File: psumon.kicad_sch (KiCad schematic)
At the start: 4 parts, among them U1 INA260

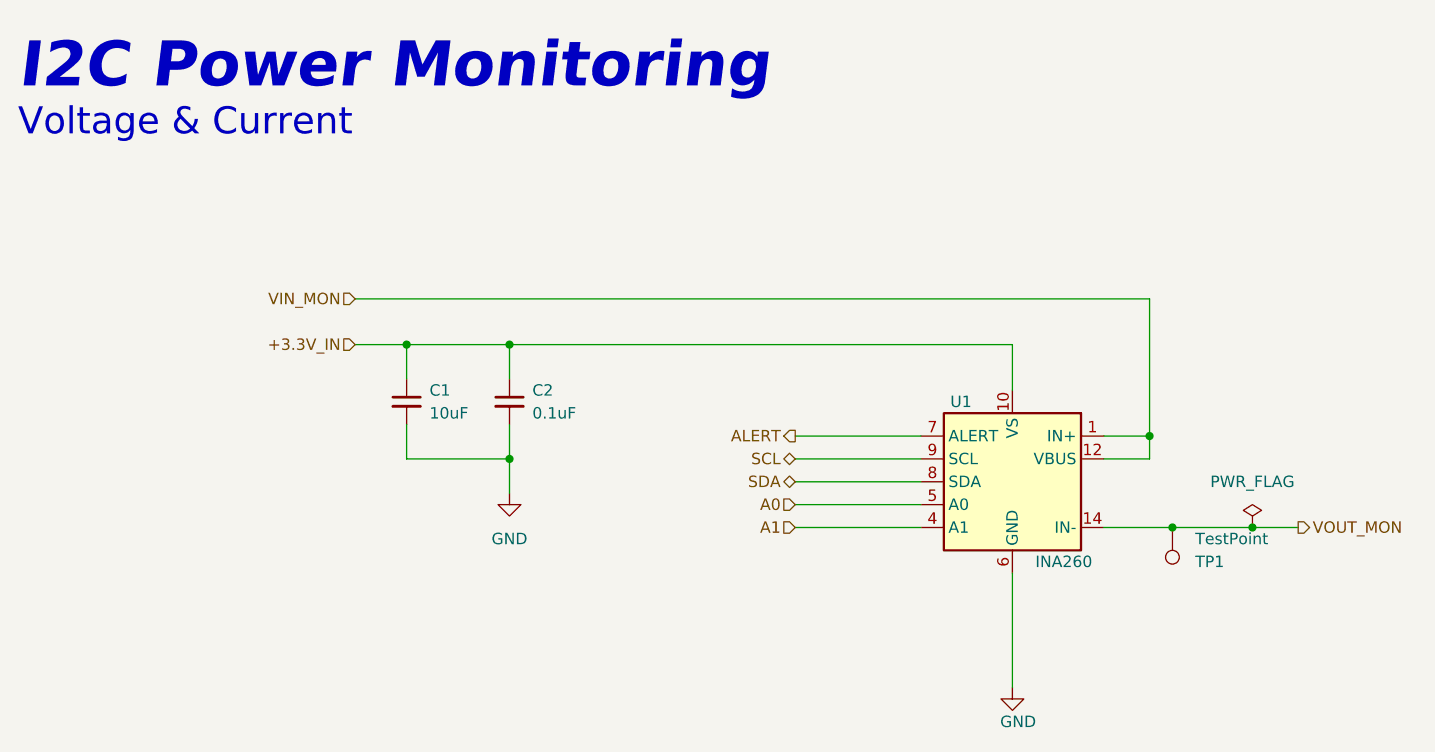
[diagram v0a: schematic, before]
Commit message: leds
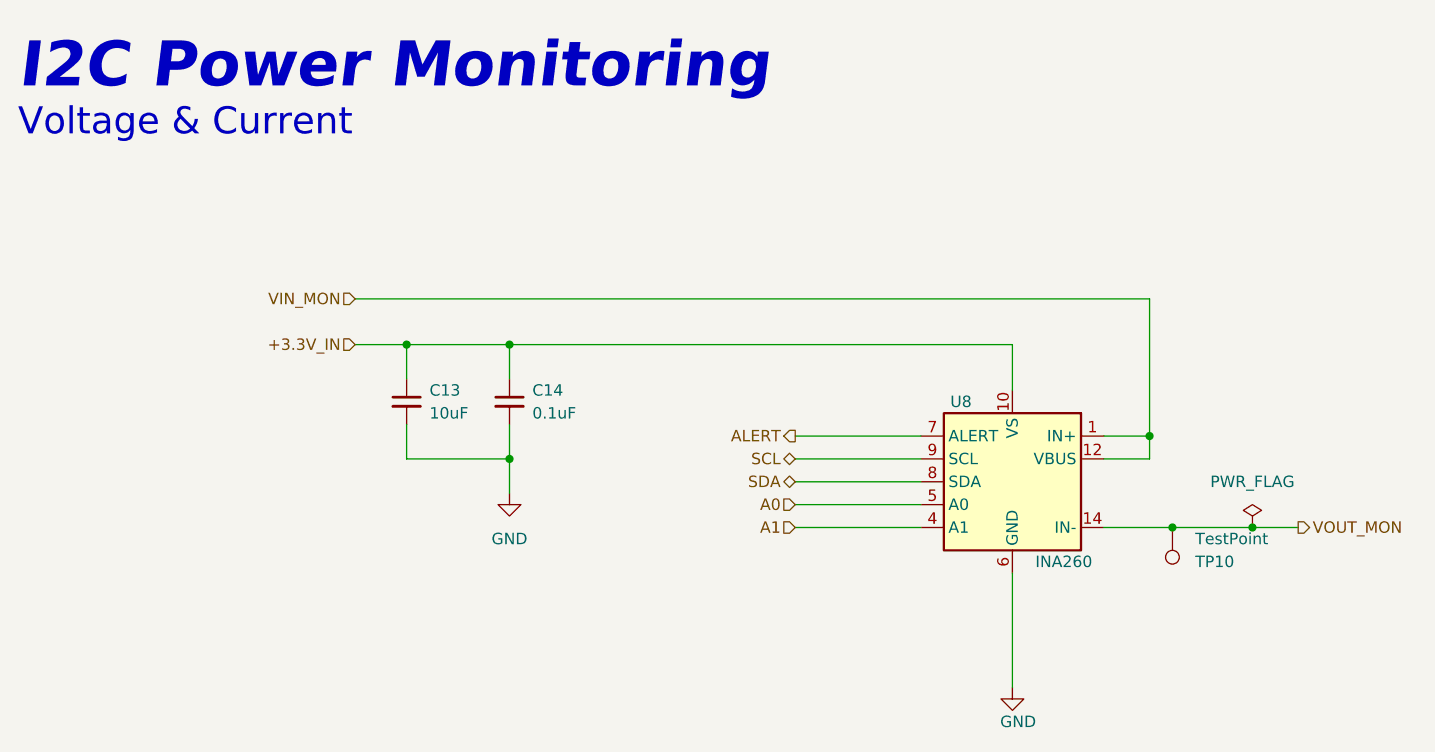
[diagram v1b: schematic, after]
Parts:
- renumbered C1 to C13, C2 to C14, TP1 to TP10, U1 to U8
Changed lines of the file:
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@@
   (symbol (lib_id "power:GND") (at 125.73 90.17 0)
     (in_bom yes) (on_board yes)
-    (property "Reference" "#PWR03" (id 0) (at 125.73 96.52 0)
+    (property "Reference" "#PWR023" (id 0) (at 125.73 96.52 0)
       (effects (font (size 1.27 1.27)) hide)
     )
@@
   (symbol (lib_id "Device:C_Small") (at 58.42 58.42 0)
     (in_bom yes) (on_board yes) (fields_autoplaced)
-    (property "Reference" "C1" (id 0) (at 60.96 57.1562 0)
+    (property "Reference" "C13" (id 0) (at 60.96 57.1562 0)
       (effects (font (size 1.27 1.27)) (justify left))
     )
@@
   (symbol (lib_id "power:GND") (at 69.85 68.58 0)
     (in_bom yes) (on_board yes) (fields_autoplaced)
-    (property "Reference" "#PWR02" (id 0) (at 69.85 74.93 0)
+    (property "Reference" "#PWR022" (id 0) (at 69.85 74.93 0)
       (effects (font (size 1.27 1.27)) hide)
     )
@@
   (symbol (lib_id "Sensor_I2C_TI:INA260") (at 125.73 67.31 0) (mirror y)
     (in_bom yes) (on_board yes)
-    (property "Reference" "U1" (id 0) (at 120.015 58.42 0))
+    (property "Reference" "U8" (id 0) (at 120.015 58.42 0))
     (property "Value" "INA260" (id 1) (at 131.445 76.2 0))
     (property "Footprint" "Sensor_I2C_TI:TSSOP-16_4.4x5mm_P0.65mm_pin1" (id 2) (at 124.46 99.06 0)
@@
   (symbol (lib_id "power:PWR_FLAG") (at 152.4 72.39 0)
     (in_bom yes) (on_board yes) (fields_autoplaced)
-    (property "Reference" "#FLG03" (id 0) (at 152.4 70.485 0)
+    (property "Reference" "#FLG04" (id 0) (at 152.4 70.485 0)
       (effects (font (size 1.27 1.27)) hide)
     )
@@
   (symbol (lib_id "Device:C_Small") (at 69.85 58.42 0)
     (in_bom yes) (on_board yes) (fields_autoplaced)
-    (property "Reference" "C2" (id 0) (at 72.39 57.1562 0)
+    (property "Reference" "C14" (id 0) (at 72.39 57.1562 0)
       (effects (font (size 1.27 1.27)) (justify left))
     )
@@
   (symbol (lib_id "Connector:TestPoint") (at 143.51 72.39 0) (mirror x)
     (in_bom yes) (on_board yes)
-    (property "Reference" "TP1" (id 0) (at 146.05 76.2 0)
+    (property "Reference" "TP10" (id 0) (at 146.05 76.2 0)
       (effects (font (size 1.27 1.27)) (justify left))
     )
